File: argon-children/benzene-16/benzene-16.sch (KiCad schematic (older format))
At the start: 17 parts, among them U1 Conn1, U2 SPI FLASH, U3 Conn2, U4 LMC555, U5 IS25WP256D-xM

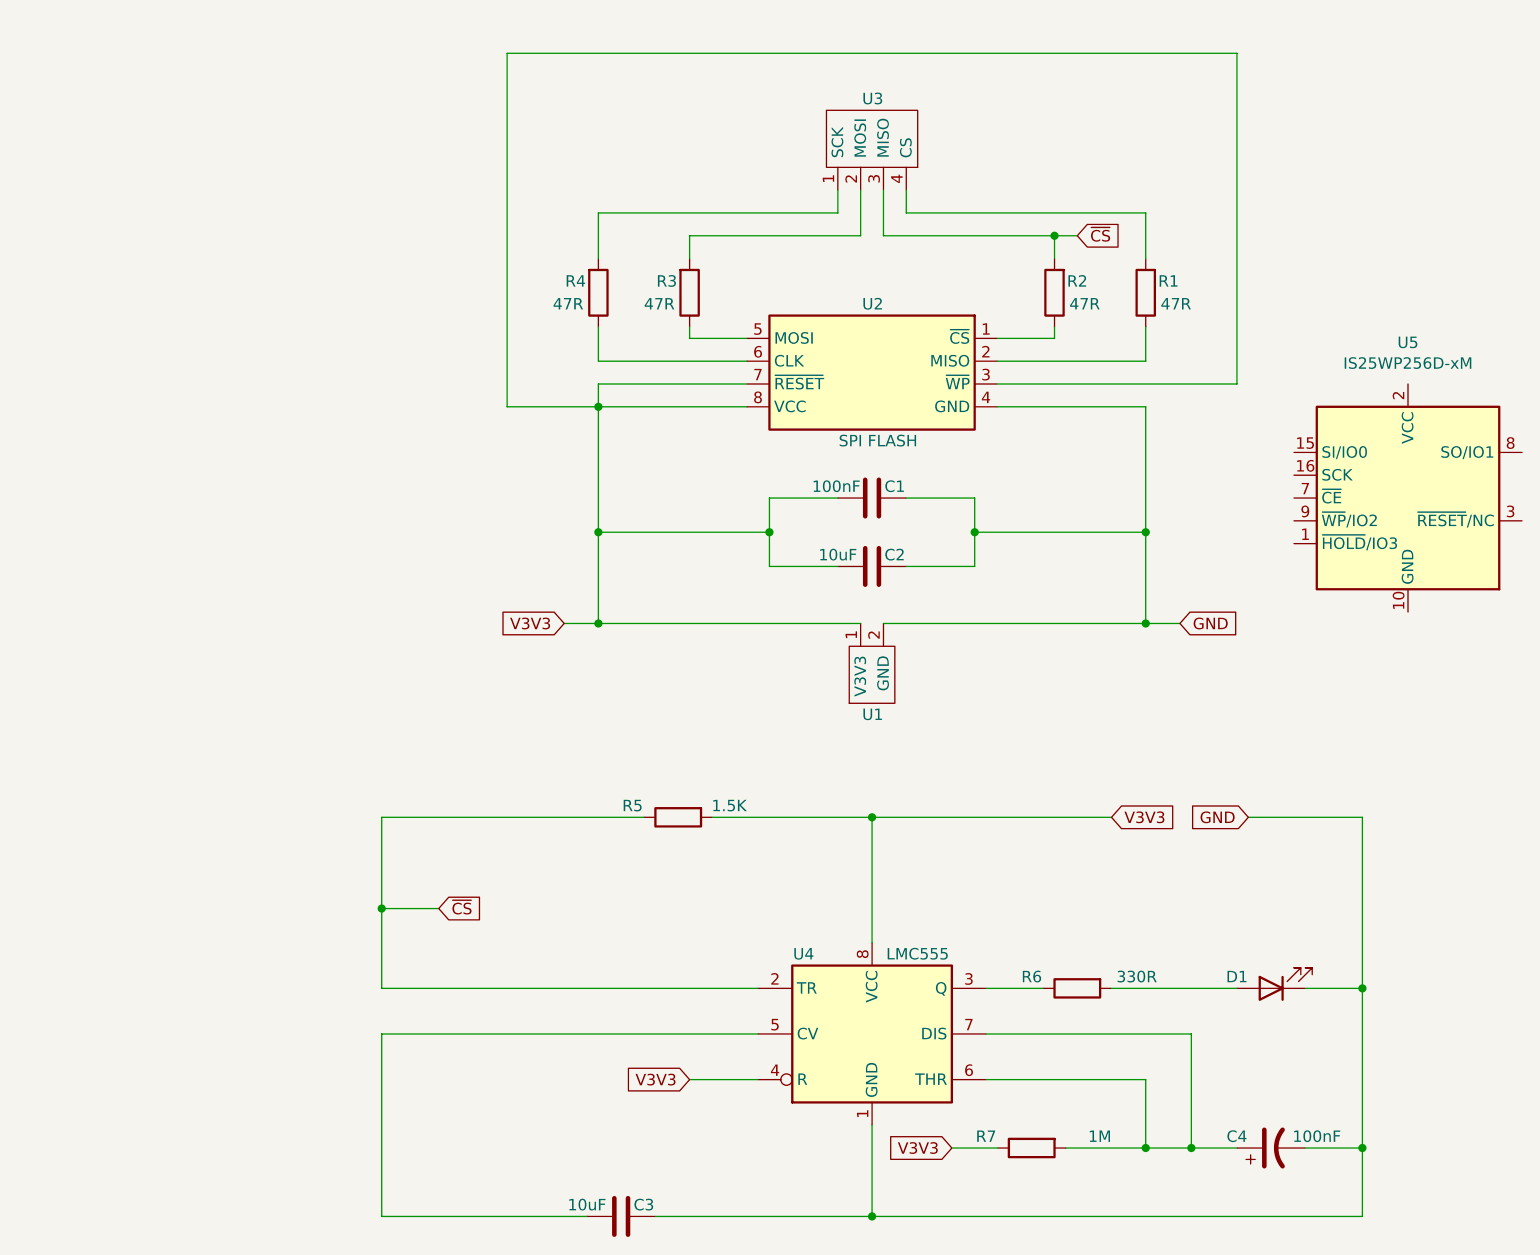
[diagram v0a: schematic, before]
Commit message: Benzene schematic
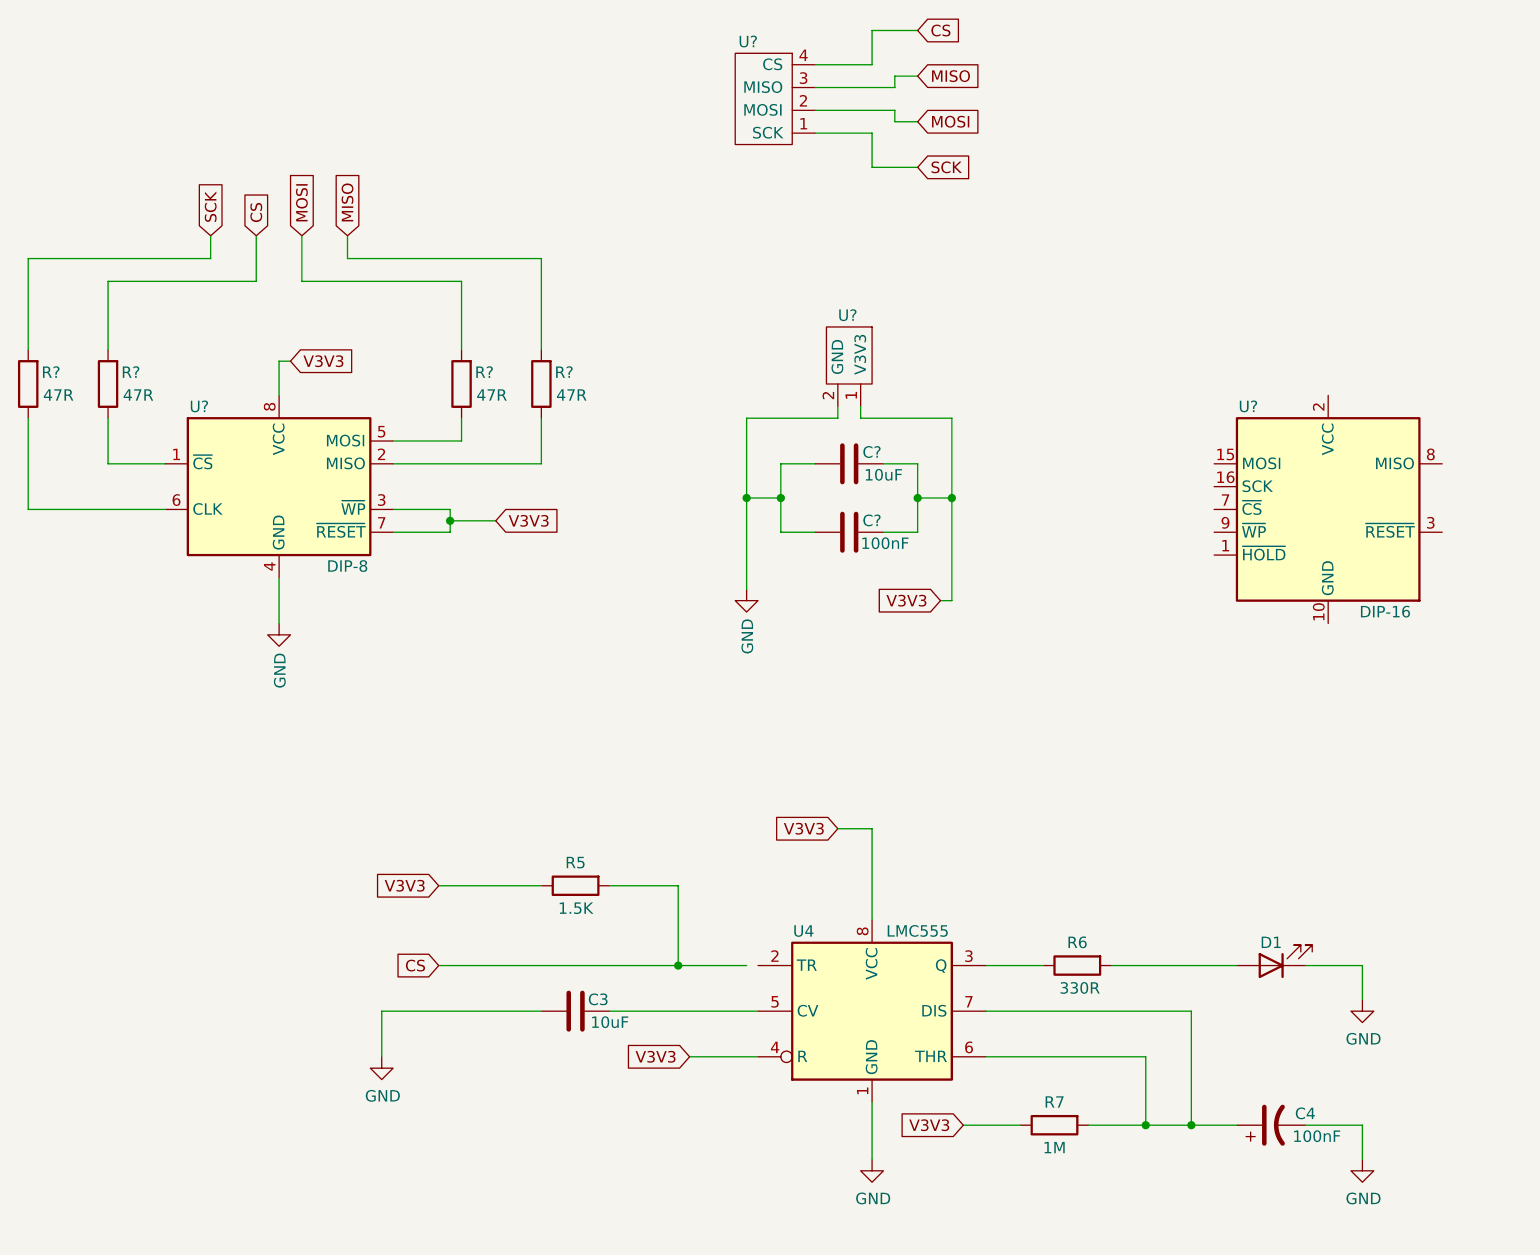
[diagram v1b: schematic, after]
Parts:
- removed C1: 100nF, Capacitor_SMD:C_0603_1608Metric, symbol Device:C
- removed C2: 10uF, Capacitor_SMD:C_0603_1608Metric, symbol Device:C
- removed R1, R2, R3, R4: 47R, Resistor_SMD:R_0603_1608Metric, symbol Device:R
- removed U1: Conn1, Connector_PinHeader_2.54mm:PinHeader_1x02_P2.54mm_Vertical, symbol ArgonComponents:Conn1
- removed U2: SPI FLASH, benzene:DIP-8_W7.62mm_Socket, symbol ArgonComponents:SPI_FLASH
- removed U3: Conn2, Connector_PinHeader_2.54mm:PinHeader_1x04_P2.54mm_Vertical, symbol ArgonComponents:Conn2
- removed U5: IS25WP256D-xM, benzene:DIP-16_W15.24mm, symbol Memory_Flash:IS25WP256D-xM
- added C?: 100nF, Capacitor_SMD:C_0603_1608Metric, symbol Device:C
- added C?: 10uF, Capacitor_SMD:C_0603_1608Metric, symbol Device:C
- added R? (x4): 47R, Resistor_SMD:R_0603_1608Metric, symbol Device:R
- added U?: DIP-8, Package_SO:SOIC-8_5.23x5.23mm_P1.27mm, symbol ArgonComponents:spi_flash_dip_8
- added U?: DIP-16, Package_SO:SOIC-16W_7.5x10.3mm_P1.27mm, symbol ArgonComponents:spi_flash_dip_16
- added U?: Conn1, Connector_PinHeader_2.54mm:PinHeader_1x02_P2.54mm_Vertical, symbol ArgonComponents:Conn1
- added U?: Conn2, Connector_PinHeader_2.54mm:PinHeader_1x04_P2.54mm_Vertical, symbol ArgonComponents:Conn2
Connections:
- net GND: now also C3.1, C?.2, C?.2, U?.2 (GND), U?.4 (GND); no longer C3.2
- net V3V3: now also R5.1, C?.1, C?.1, U?.1 (V3V3), U?.3 (~WP), U?.7 (~RESET), U?.8 (VCC); no longer R5.2
- net at U4.5 (CV): now also C3.2; no longer C3.1
- net ~CS: no longer names the net of U4.2 (TR)
- net ~CS: no longer R5.1
- new net: R?.1, U?.1 (~CS)
- new net: R?.1, U?.2 (MISO)
- new net: R?.1, U?.5 (MOSI)
- new net: R?.1, U?.6 (CLK)
- new net CS: R5.2, R?.2, U?.4 (CS)
- new net MISO: R?.2, U?.3 (MISO)
- new net MOSI: R?.2, U?.2 (MOSI)
- new net SCK: R?.2, U?.1 (SCK)
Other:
- moved on the sheet: C3, C4, D1, R5, R6, R7, U4
